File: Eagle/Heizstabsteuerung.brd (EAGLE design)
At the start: 100 x 80 mm, 17 parts, among them U1 ESP32-DEVKITC-32D, X1 JST-XH-03-PIN-ROUND-PAD, X2 JST-XH-03-PIN-ROUND-PAD, X3 JST-XH-03-PIN-ROUND-PAD, X4 Versorgung

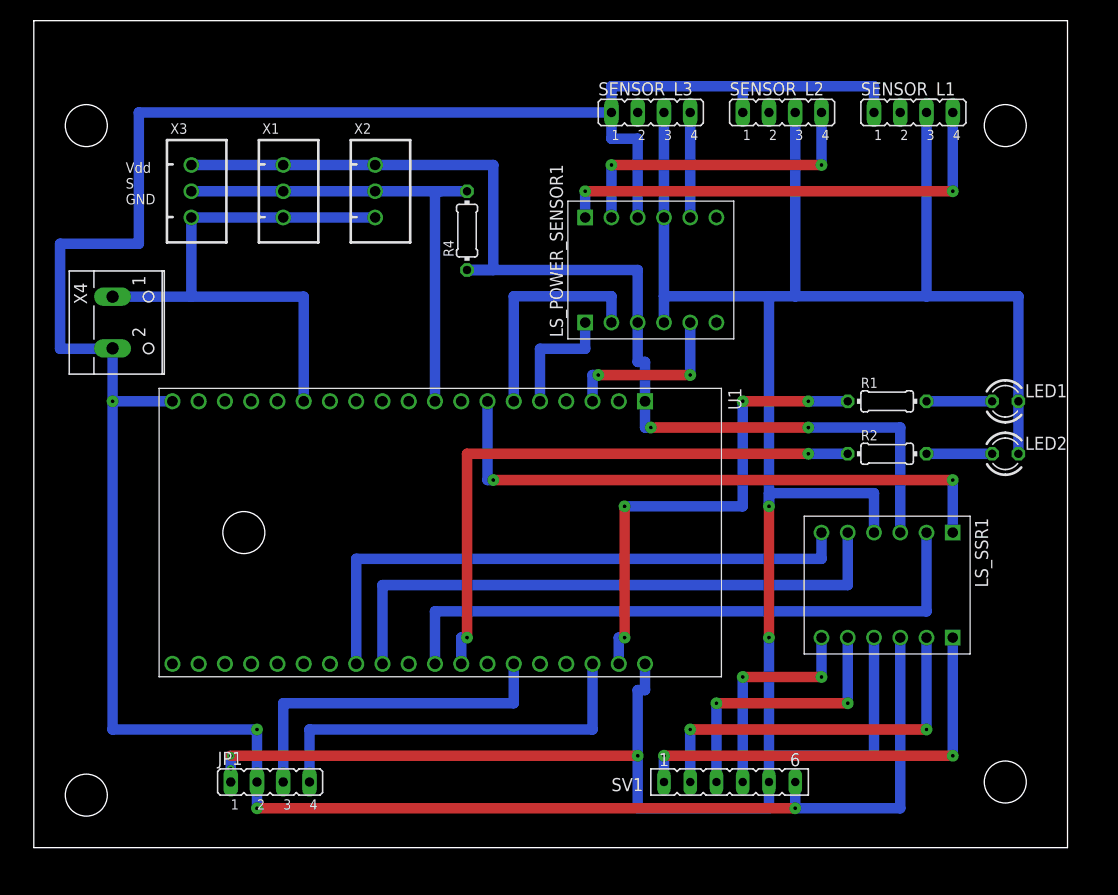
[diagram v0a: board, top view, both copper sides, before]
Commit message: Update V2.02 übertragen
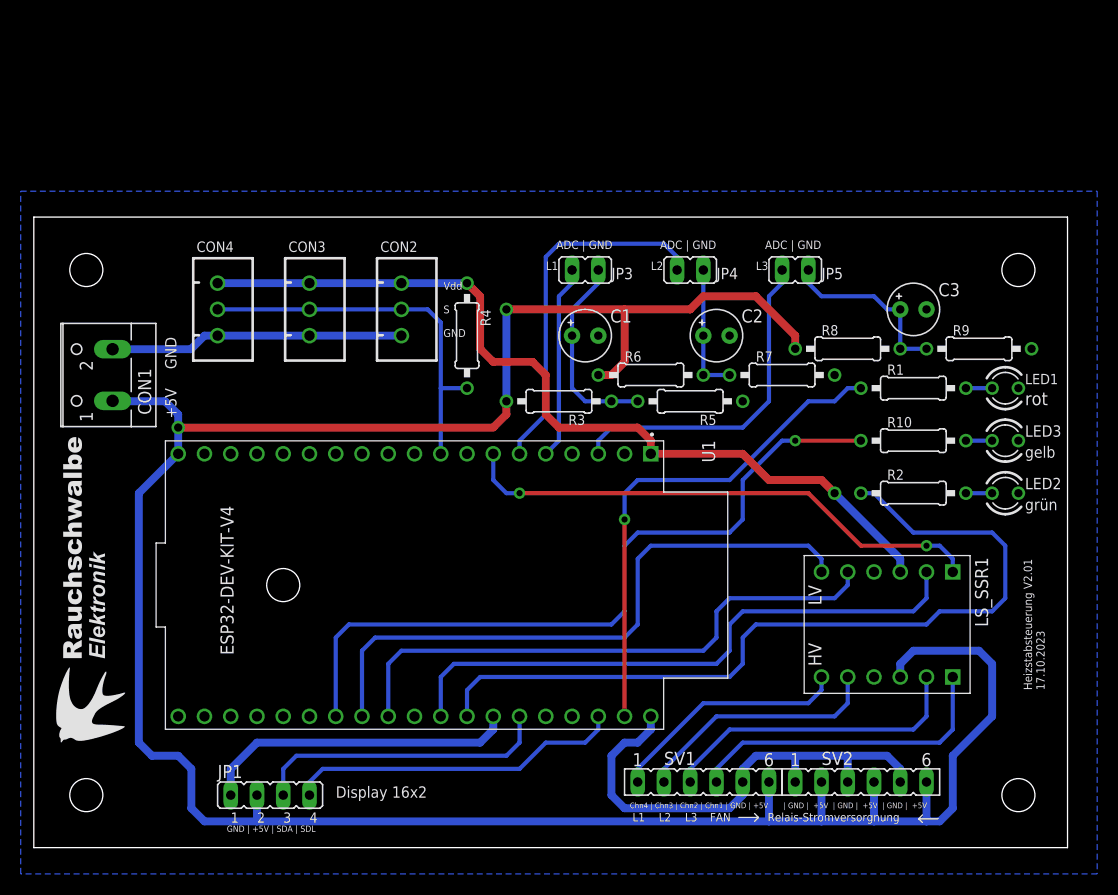
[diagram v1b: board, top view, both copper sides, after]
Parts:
- removed LS_POWER_SENSOR1: BOB-12009, BOB-12009:CONV_BOB-12009
- removed SENSOR_L1, SENSOR_L2, SENSOR_L3: (no value), jumper:JP4
- removed X1, X2, X3: JST-XH-03-PIN-ROUND-PAD, Rembrandt Electronics - JST XH Connectors v1-0:JST-XH-03-PACKAGE-ROUND-PAD
- removed X4: Versorgung, con-wago-500:W237-102
- added C1, C2, C3: 10µF, Heizstabsteuerung:E2,5-5
- added CON1: (no value), Heizstabsteuerung:WAGO-500-2
- added CON2, CON3, CON4: JST-XH-03, Heizstabsteuerung:JST-XH-03
- added JP3: L1, jumper:JP1
- added JP4: L2, jumper:JP1
- added JP5: L3, jumper:JP1
- added LED3: gelb, Heizstabsteuerung:LED3MM
- added R10: 220, Heizstabsteuerung:0207/10
- added R3, R5, R6, R7, R8, R9: 10k, Heizstabsteuerung:0207/10
- added SV2: (no value), Heizstabsteuerung:FE06
- added U$1: LOGO_RAUCHSCHWALBE, Heizstabsteuerung:LOGO_RAUCHSCHWALBE
- JP1: value Display -> Display 16x2
- LED1: value red -> rot; device led:LED3MM -> Heizstabsteuerung:LED3MM
- LED2: device led:LED3MM -> Heizstabsteuerung:LED3MM
- LS_SSR1: value BOB-12009 -> LEVELSHIFTER; device BOB-12009:CONV_BOB-12009 -> Heizstabsteuerung:LEVELSHIFTER
- R1, R4: device rcl:0204/7 -> Heizstabsteuerung:0207/10
- R2: value 220 -> 330; device rcl:0204/7 -> Heizstabsteuerung:0207/10
- SV1: device con-lsta:FE06 -> Heizstabsteuerung:FE06
- U1: value ESP32-DEVKITC-32D -> ESP32-DEV-KIT-V4; device ESP32-DEVKITC-32D:MODULE_ESP32-DEVKITC-32D -> Heizstabsteuerung:ESP32-DEV-KIT-V4
- moved R4 10.2 mm to (41.9, 49.5), turned to 270 degrees
- moved U1 5.68 mm to (36.8, 25.4)
- moved R2 4.58 mm to (85.1, 34.3)
- moved LED2 3.81 mm to (94.0, 34.3)
- moved LS_SSR1 3.81 mm to (82.5, 21.6)
- moved R1 2.84 mm to (85.1, 44.5)
- moved SV1 2.54 mm to (64.8, 6.35)
- moved LED1 1.27 mm to (94.0, 44.5)
- moved JP1 1.27 mm to (22.9, 5.08)
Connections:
- removed net GND$2: JP1.1, LED1.K, LED2.K, LS_POWER_SENSOR1.GND_1, LS_POWER_SENSOR1.GND_2, LS_SSR1.GND_1, LS_SSR1.GND_2, SENSOR_L1.3, SENSOR_L2.3, SENSOR_L3.3, SV1.5, U1.14, U1.20, U1.26, X1.3, X2.3, X3.3, X4.1
- removed net N$24: LS_POWER_SENSOR1.HV3, SENSOR_L3.4
- removed net N$25: LS_POWER_SENSOR1.HV2, SENSOR_L2.4
- removed net N$26: LS_POWER_SENSOR1.HV1, SENSOR_L1.4
- removed net VDD3$13: LS_POWER_SENSOR1.LV, LS_SSR1.LV, R4.1, U1.1, X1.1, X2.1, X3.1
- removed net VDD5$3: JP1.2, LS_POWER_SENSOR1.HV, LS_SSR1.HV, SENSOR_L1.1, SENSOR_L2.1, SENSOR_L3.1, SV1.6, U1.19, X4.2
- new net +3V3: CON2.1, CON3.1, CON4.1, LS_SSR1.LV, R4.1, U1.1
- new net +5V: CON1.1, JP1.2, LS_SSR1.HV, R3.1, R6.1, R8.1, SV1.6, SV2.2, SV2.4, SV2.6, U1.19
- new net GND: C1.-, C2.-, C3.-, CON1.2, CON2.3, CON3.3, CON4.3, JP1.1, LED1.K, LED2.K, LED3.K, LS_SSR1.GND_1, LS_SSR1.GND_2, R5.2, R7.2, R9.2, SV1.5, SV2.1, SV2.3, SV2.5, U1.14, U1.32, U1.38
- new net N$17: R10.1, U1.26
- new net N$2: C1.+, JP3.2, R3.2, R5.1
- new net N$27: C2.+, JP4.2, R6.2, R7.1
- new net N$28: C3.+, JP5.2, R8.2, R9.1
- new net N$3: LED3.A, R10.2
- net N$1: now also U1.37; no longer U1.21
- net N$11: now also CON2.2, CON3.2, CON4.2; no longer X1.2, X2.2, X3.2
- net N$12: now also JP3.1; no longer LS_POWER_SENSOR1.LV1
- net N$14: now also U1.27; no longer U1.31
- net N$15: now also U1.28; no longer U1.30
- net N$16: now also U1.30; no longer U1.28
- net N$18: now also SV1.4; no longer SV1.1
- net N$19: now also SV1.3; no longer SV1.2
- net N$20: now also SV1.2; no longer SV1.3
- net N$21: now also JP4.1; no longer LS_POWER_SENSOR1.LV2
- net N$22: now also JP5.1; no longer LS_POWER_SENSOR1.LV3
- net N$4: now also U1.33; no longer U1.25
- net N$5: now also U1.36; no longer U1.22
- net N$6: now also U1.31; no longer U1.27
- net N$9: now also SV1.1; no longer SV1.4
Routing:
- net GND$2: track 315.1 -> 0.00 mm, vias 5 -> 0
- net VDD5$3: track 272.6 -> 0.00 mm, vias 4 -> 0
- net +5V: track 0.00 -> 251.3 mm, vias 0 -> 2
- net VDD3$13: track 109.2 -> 0.00 mm, vias 2 -> 0
- net GND: track 0.00 -> 108.1 mm
- net +3V3: track 0.00 -> 84.3 mm, vias 0 -> 1
- net N$17: track 0.00 -> 72.3 mm, vias 0 -> 1
- net N$26: track 45.7 -> 0.00 mm, vias 2 -> 0
- net N$25: track 30.5 -> 0.00 mm, vias 2 -> 0
- net N$6: track 57.7 -> 80.9 mm, vias 2 -> 0
- net N$2: track 0.00 -> 19.4 mm
- net N$28: track 0.00 -> 17.6 mm
- net N$22: track 17.1 -> 32.6 mm, vias 2 -> 0
- net N$21: track 22.2 -> 35.1 mm
- net N$27: track 0.00 -> 12.7 mm
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- added copper zone on layer 16, net GND
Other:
- board size 100 x 80 mm -> 100 x 61 mm
- board text added: "ADC | GND"
- board text added: "FAN"
- board text added: "Heizstabsteuerung V2.01 17.10.2023"
- board text added: "L1"
- board text added: "L2"
- board text added: "L3"
- board text added: "Relais-Stromversorgnung"
- board text added: "| GND | +5V | GND | +5V | GND | +5V"
- board text removed: "5V | NC | GND | Sig"
